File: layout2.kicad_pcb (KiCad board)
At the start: 2 copper layers, 68.6 x 53.3 mm, 12 parts, among them J1 Conn_01x08_Female, P1 Power, P2 Analog, P3 Digital, P4 Digital, P5 CONN_01X01, P6 CONN_01X01, P7 CONN_01X01, P8 CONN_01X01, U1 Capteur_AIME, U2 LTC1100xN8

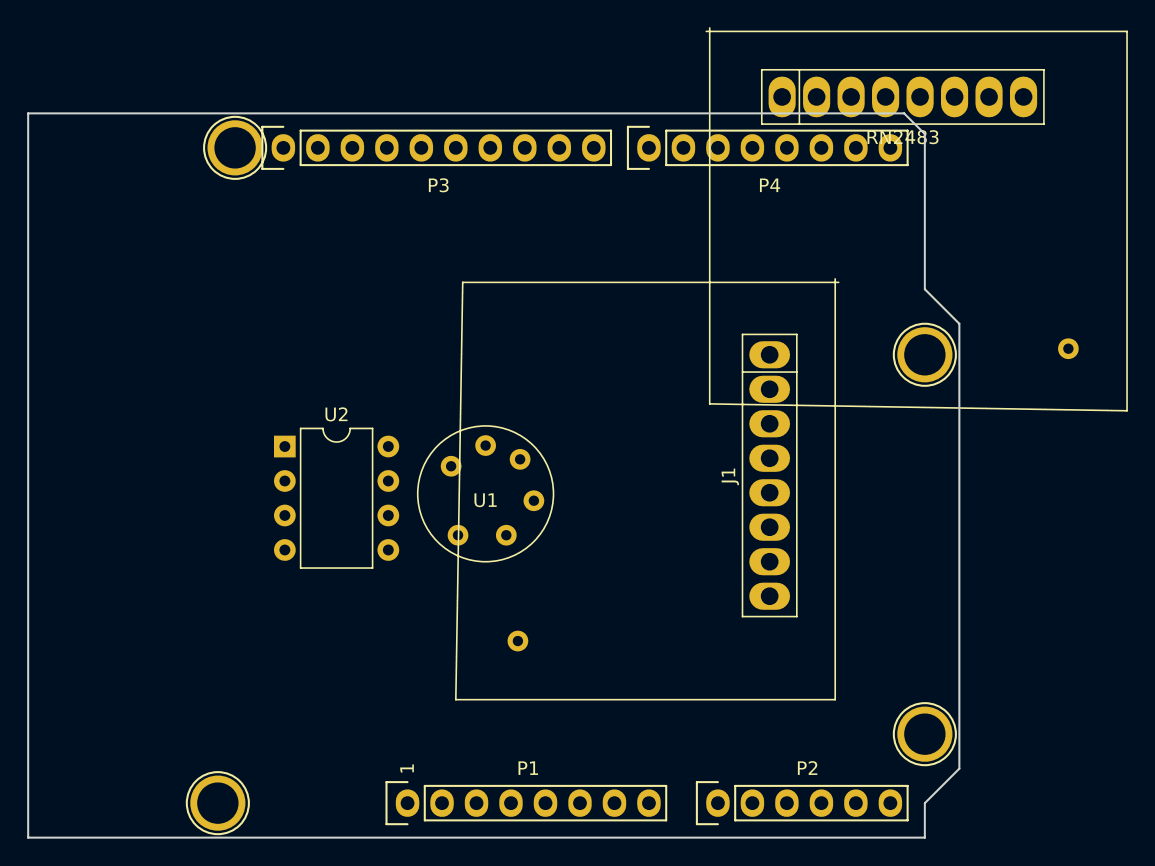
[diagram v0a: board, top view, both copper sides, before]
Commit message: Final push
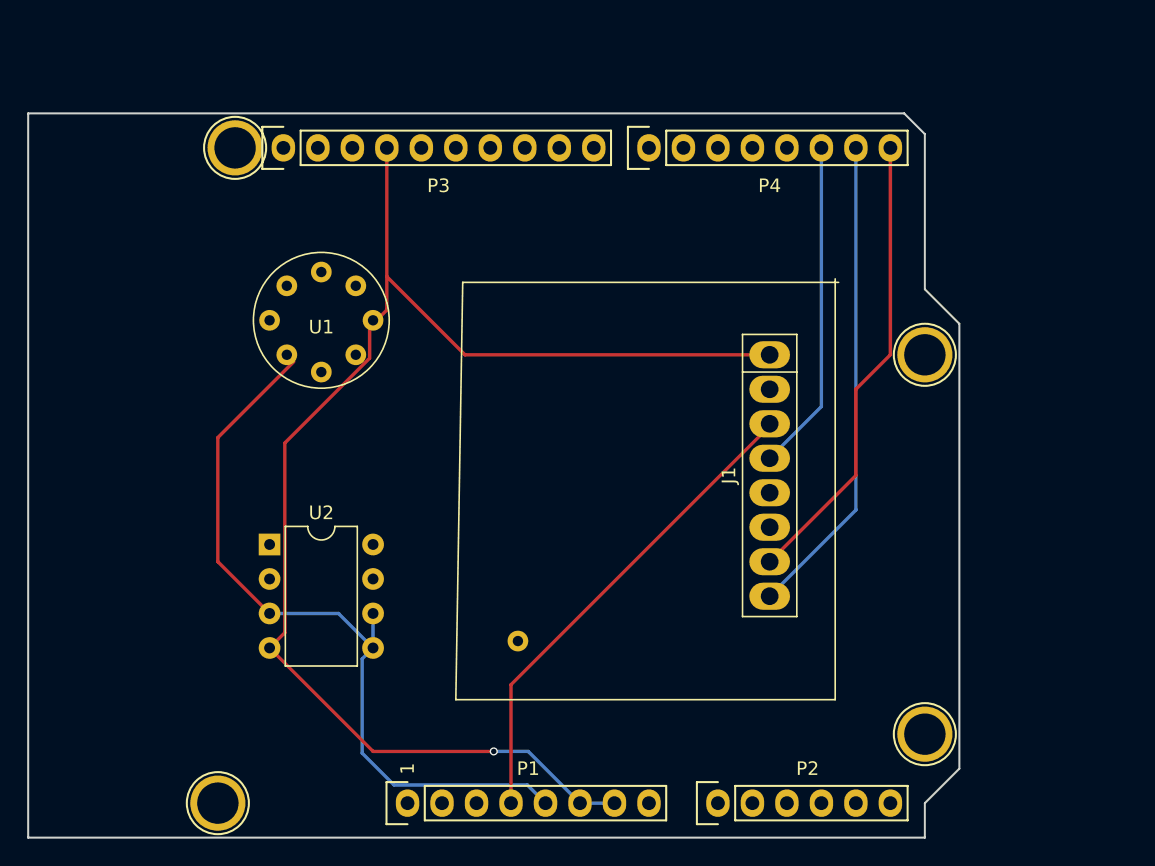
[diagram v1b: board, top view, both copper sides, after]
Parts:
- removed RN2483: Lora, Capteur_AIME:RN2483_new
- moved U1 17.6 mm to (132.6, 88.3)
- moved U2 7.30 mm to (128.8, 104.8)
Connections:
- J1 pad 4: Net-(J1-Pad4) -> /2
- J1 pad 7: Net-(J1-Pad7) -> /0(Rx)
- J1 pad 8: Net-(J1-Pad8) -> /1(Tx)
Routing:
- net GND: track 0.00 -> 101.1 mm, vias 0 -> 2
- net +5V: track 0.00 -> 56.7 mm
- net +3V3: track 0.00 -> 36.1 mm
- net /1(Tx): track 0.00 -> 35.7 mm
- net /0(Rx): track 0.00 -> 34.2 mm
- net /2: track 0.00 -> 24.4 mm
